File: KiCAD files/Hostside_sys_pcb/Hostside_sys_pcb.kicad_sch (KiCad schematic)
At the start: 8 parts, among them U1 L7805, U2 Pico

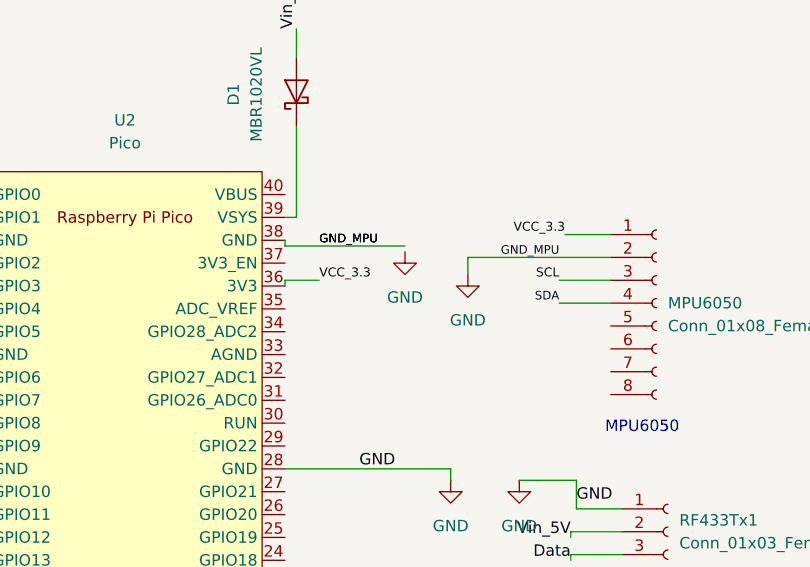
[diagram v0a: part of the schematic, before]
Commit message: Hostside kicad files updated and added
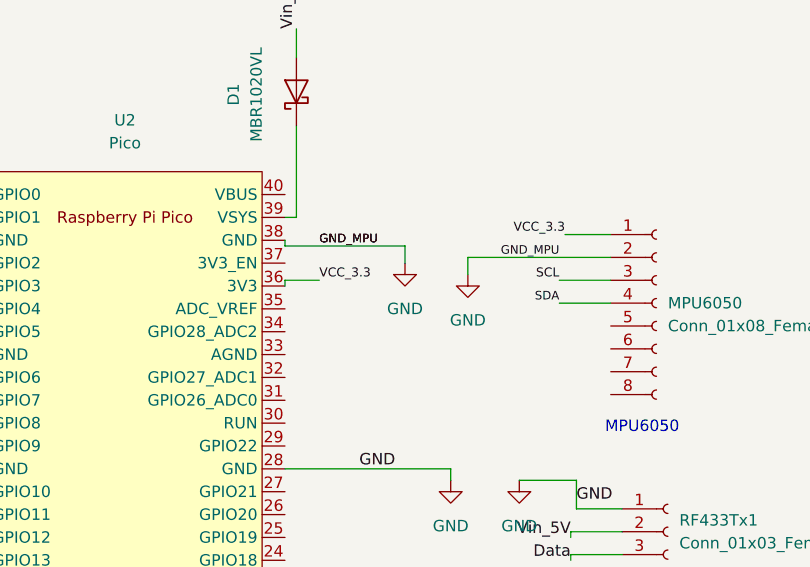
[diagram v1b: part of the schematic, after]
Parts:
- C1, C2: footprint Capacitor_THT:CP_Radial_D5.0mm_P2.00mm -> Capacitor_THT:CP_Radial_D5.0mm_P2.50mm
- D1: footprint Diode_THT:D_A-405_P7.62mm_Horizontal -> Diode_THT:D_A-405_P2.54mm_Vertical_KathodeUp
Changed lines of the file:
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@@
+    (stroke (width 0) (type default) (color 0 0 0 0))
+  )
+  (wire (pts (xy 202.565 67.945) (xy 202.565 69.85))
     (stroke (width 0) (type default) (color 0 0 0 0))
   )
@@
     (pin "1")
   )
-  (symbol (lib_id "power:GND") (at 202.565 68.58 0) (unit 1)
-    (in_bom yes) (on_board yes) (fields_autoplaced)
-    (property "Reference" "#PWR0105" (id 0) (at 202.565 74.93 0)
-      (effects (font (size 1.27 1.27)) hide)
-    )
-    (property "Value" "GND" (id 1) (at 202.565 73.66 0))
-    (property "Footprint" "" (id 2) (at 202.565 68.58 0)
-      (effects (font (size 1.27 1.27)) hide)
-    )
-    (property "Datasheet" "" (id 3) (at 202.565 68.58 0)
+  (symbol (lib_id "power:GND") (at 202.565 69.85 0) (unit 1)
+    (in_bom yes) (on_board yes) (fields_autoplaced)
+    (property "Reference" "#PWR0105" (id 0) (at 202.565 76.2 0)
+      (effects (font (size 1.27 1.27)) hide)
+    )
+    (property "Value" "GND" (id 1) (at 202.565 74.93 0))
+    (property "Footprint" "" (id 2) (at 202.565 69.85 0)
+      (effects (font (size 1.27 1.27)) hide)
+    )
+    (property "Datasheet" "" (id 3) (at 202.565 69.85 0)
       (effects (font (size 1.27 1.27)) hide)
     )
@@
       (effects (font (size 1.27 1.27)) (justify left))
     )
-    (property "Footprint" "Capacitor_THT:CP_Radial_D5.0mm_P2.00mm" (id 2) (at 126.6952 92.71 0)
+    (property "Footprint" "Capacitor_THT:CP_Radial_D5.0mm_P2.50mm" (id 2) (at 126.6952 92.71 0)
       (effects (font (size 1.27 1.27)) hide)
     )
@@
     (property "Reference" "D1" (id 0) (at 183.515 51.1175 0))
     (property "Value" "MBR1020VL" (id 1) (at 186.055 51.1175 0))
-    (property "Footprint" "Diode_THT:D_A-405_P7.62mm_Horizontal" (id 2) (at 194.945 50.8 0)
+    (property "Footprint" "Diode_THT:D_A-405_P2.54mm_Vertical_KathodeUp" (id 2) (at 194.945 50.8 0)
       (effects (font (size 1.27 1.27)) hide)
     )
@@
       (effects (font (size 1.27 1.27)) (justify left))
     )
-    (property "Footprint" "Capacitor_THT:CP_Radial_D5.0mm_P2.00mm" (id 2) (at 77.1652 85.09 0)
+    (property "Footprint" "Capacitor_THT:CP_Radial_D5.0mm_P2.50mm" (id 2) (at 77.1652 85.09 0)
       (effects (font (size 1.27 1.27)) hide)
     )
@@
     )
     (path "/b48e6e0f-13df-49a2-b441-8b6960c65029"
-      (reference "C1") (unit 1) (value "C") (footprint "Capacitor_THT:CP_Radial_D5.0mm_P2.00mm")
+      (reference "C1") (unit 1) (value "C") (footprint "Capacitor_THT:CP_Radial_D5.0mm_P2.50mm")
     )
     (path "/414f0eb4-bfc6-42f4-9c12-4522d3366a4e"
-      (reference "C2") (unit 1) (value "C") (footprint "Capacitor_THT:CP_Radial_D5.0mm_P2.00mm")
+      (reference "C2") (unit 1) (value "C") (footprint "Capacitor_THT:CP_Radial_D5.0mm_P2.50mm")
     )
     (path "/4f2b6c7f-4bf2-402e-8d97-019a6f64dd80"
-      (reference "D1") (unit 1) (value "MBR1020VL") (footprint "Diode_THT:D_A-405_P7.62mm_Horizontal")
+      (reference "D1") (unit 1) (value "MBR1020VL") (footprint "Diode_THT:D_A-405_P2.54mm_Vertical_KathodeUp")
     )
     (path "/9f104f48-f40b-4f13-9bc3-9168611e201a"
